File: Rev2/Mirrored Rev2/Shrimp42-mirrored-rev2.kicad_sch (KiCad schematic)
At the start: 46 parts, among them J1 02x05, J2 02x05, U1 ProMicro, U2 trrs

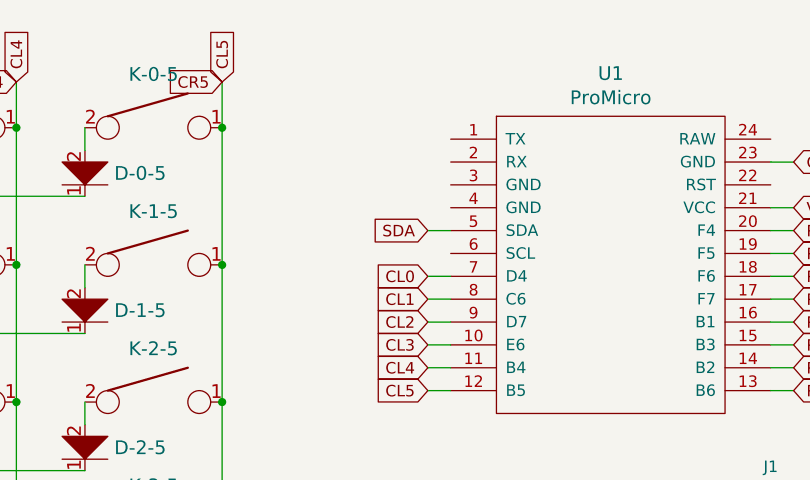
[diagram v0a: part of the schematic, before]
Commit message: rewired board. change pcb holes. push commit before order pcb
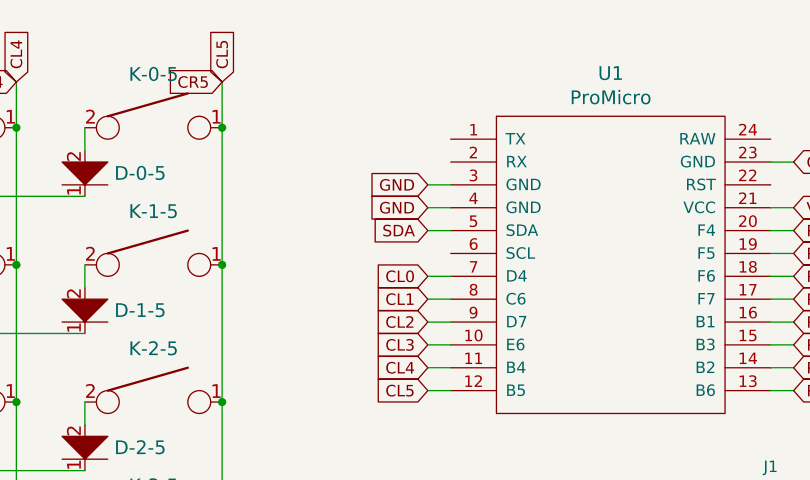
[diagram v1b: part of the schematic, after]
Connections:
- net GND: now also U1.3 (GND), U1.4 (GND)
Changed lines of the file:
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@@
+    (stroke (width 0) (type default) (color 0 0 0 0))
+  )
+  (wire (pts (xy 172.72 29.21) (xy 175.26 29.21))
     (stroke (width 0) (type default) (color 0 0 0 0))
   )
@@
   )
   (wire (pts (xy 106.68 17.78) (xy 106.68 22.86))
+    (stroke (width 0) (type default) (color 0 0 0 0))
+  )
+  (wire (pts (xy 172.72 31.75) (xy 175.26 31.75))
     (stroke (width 0) (type default) (color 0 0 0 0))
   )
@@
     )
   )
+  (global_label "GND" (shape input) (at 172.72 31.75 180) (fields_autoplaced)
+    (effects (font (size 1.27 1.27)) (justify right))
+    (property "Intersheet References" "${INTERSHEET_REFS}" (id 0) (at 166.5253 31.8294 0)
+      (effects (font (size 1.27 1.27)) (justify right) hide)
+    )
+  )
   (global_label "CL5" (shape input) (at 201.93 66.04 180) (fields_autoplaced)
     (effects (font (size 1.27 1.27)) (justify right))
@@
     )
   )
+  (global_label "GND" (shape input) (at 172.72 29.21 180) (fields_autoplaced)
+    (effects (font (size 1.27 1.27)) (justify right))
+    (property "Intersheet References" "${INTERSHEET_REFS}" (id 0) (at 166.5253 29.2894 0)
+      (effects (font (size 1.27 1.27)) (justify right) hide)
+    )
+  )
